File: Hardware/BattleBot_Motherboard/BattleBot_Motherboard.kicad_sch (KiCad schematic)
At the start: 2 parts, among them SW1 SW_Push

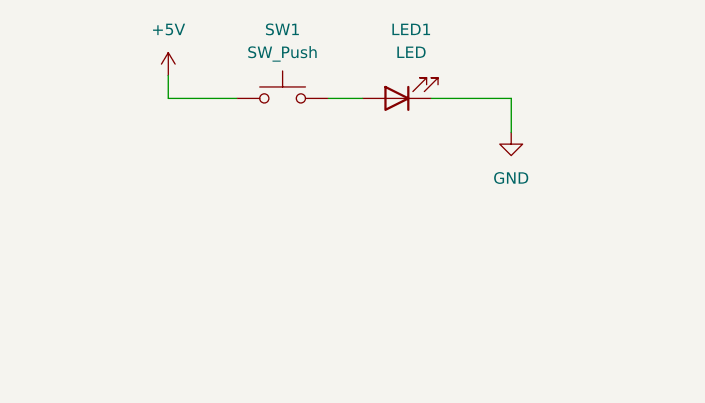
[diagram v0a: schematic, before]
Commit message: Just a cool new test thingy i made up
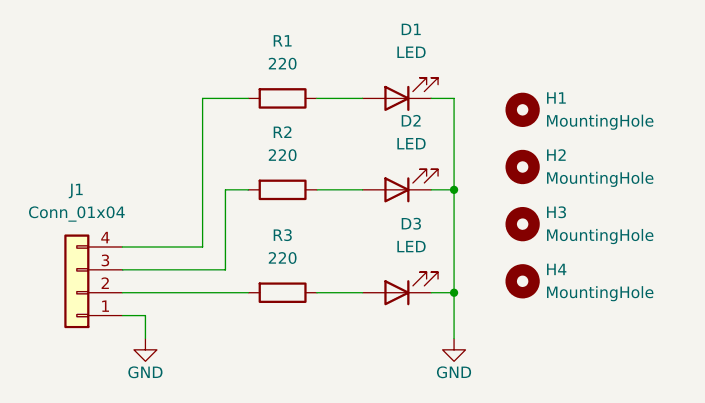
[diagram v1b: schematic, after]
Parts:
- removed SW1: SW_Push, symbol Switch:SW_Push
- added D2, D3: LED, LED_THT:LED_D3.0mm, symbol Device:LED
- added H1, H2, H3, H4: MountingHole, MountingHole:MountingHole_2.5mm_Pad, symbol Mechanical:MountingHole
- added J1: Conn_01x04, Connector_PinHeader_2.54mm:PinHeader_1x04_P2.54mm_Horizontal, symbol Connector_Generic:Conn_01x04
- added R1, R2, R3: 220, Resistor_THT:R_Axial_DIN0204_L3.6mm_D1.6mm_P5.08mm_Horizontal, symbol Device:R
- D1: renamed from LED1; footprint (none) -> LED_THT:LED_D3.0mm
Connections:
- net GND: now also D2.1 (K), D3.1 (K), J1.1 (Pin_1)
- net at D1.2 (A): now also R1.1
- new net: D2.2 (A), R2.1
- new net: J1.3 (Pin_3), R2.2
- new net: J1.2 (Pin_2), R3.2
- new net: J1.4 (Pin_4), R1.2
- new net: D3.2 (A), R3.1
